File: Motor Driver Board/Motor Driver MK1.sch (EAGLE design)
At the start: 8 parts, among them X1 MAB8SH, X2 MAB8SH, X3 MAB8SH, X4 MAB8SH

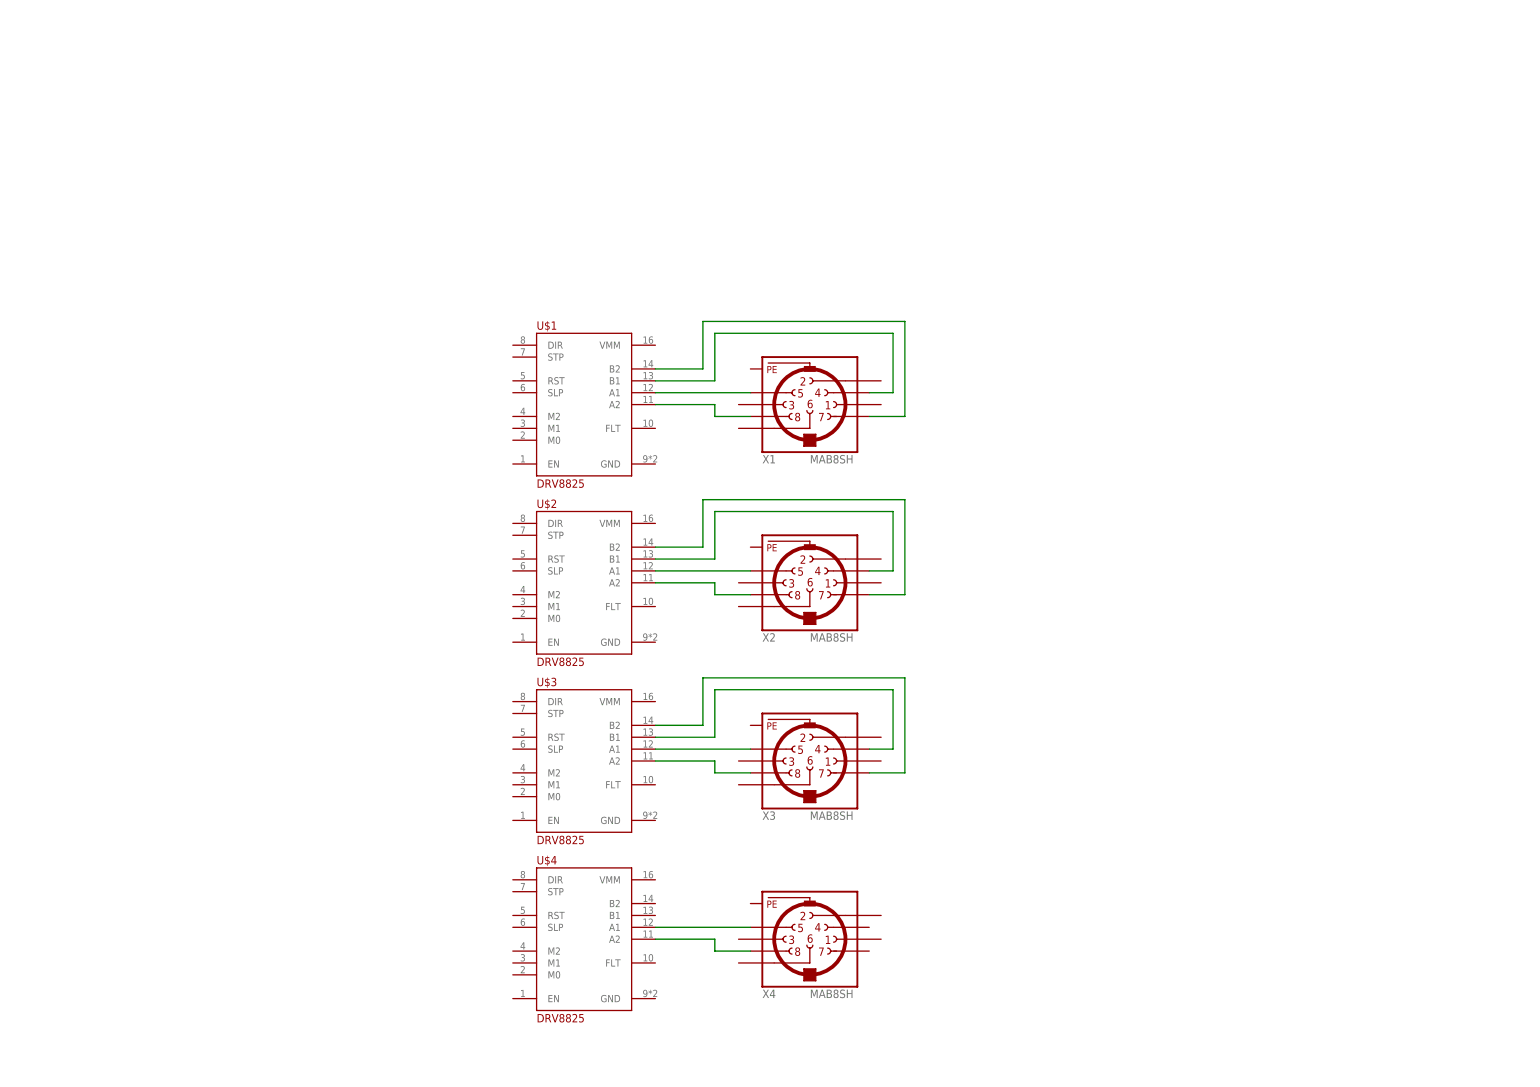
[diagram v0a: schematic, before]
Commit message: finished up schematic
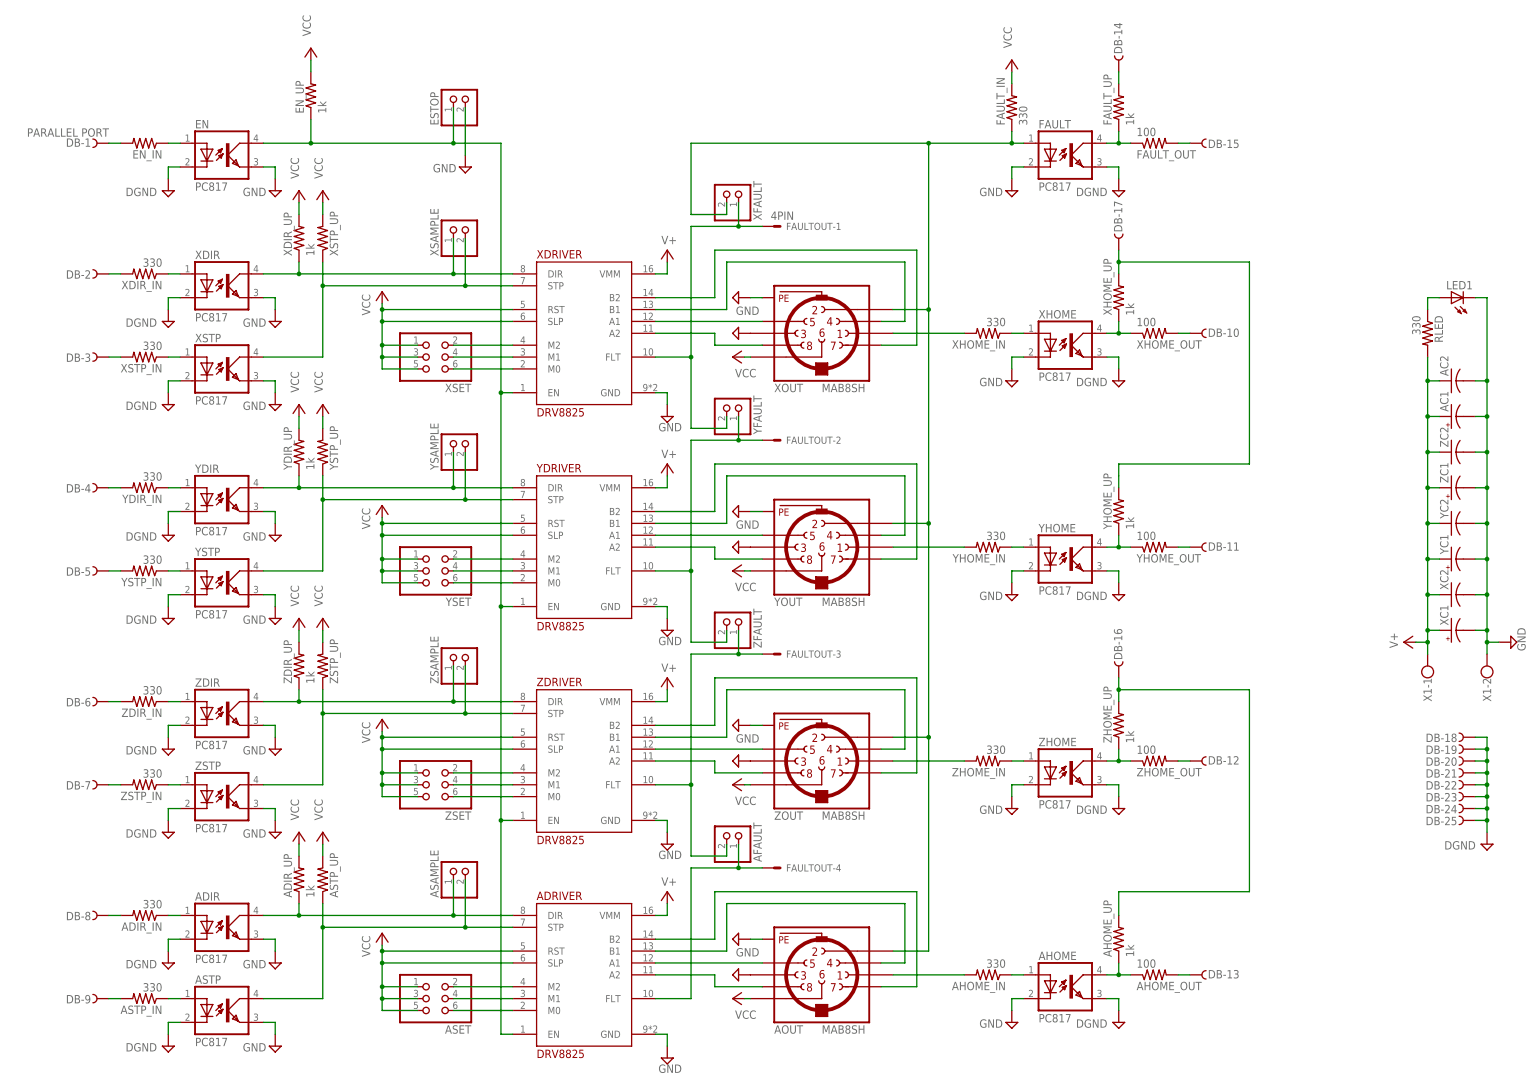
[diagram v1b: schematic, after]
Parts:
- removed U$1, U$2, U$4: DRV8825, CNC-Interface:DRV8825
- removed X2, X3, X4: MAB8SH, con-hirschmann:MAB8SH
- added AC1, XC1, YC1, ZC1: (no value), rcl:CPOL-USSANYO_SMD_F12
- added AC2, XC2, YC2, ZC2: (no value), rcl:C-USC0805
- added ADIR, AHOME, ASTP, EN, FAULT, XDIR, XHOME, XSTP, YDIR, YHOME, YSTP, ZDIR, ZHOME, ZSTP: PC817, optocoupler:PC817
- added ADIR_IN, AHOME_IN, ASTP_IN, FAULT_IN, RLED, XDIR_IN, XHOME_IN, XSTP_IN, YDIR_IN, YHOME_IN, YSTP_IN, ZDIR_IN, ZHOME_IN, ZSTP_IN: 330, resistor:R-US_R0805
- added ADIR_UP, AHOME_UP, EN_UP, FAULT_UP, XDIR_UP, XHOME_UP, YDIR_UP, YHOME_UP, ZDIR_UP, ZHOME_UP: 1k, resistor:R-US_R0805
- added ADRIVER, XDRIVER, YDRIVER: DRV8825, CNC-Interface:DRV8825
- added AFAULT, ASAMPLE, ESTOP, XFAULT, XSAMPLE, YFAULT, YSAMPLE, ZFAULT, ZSAMPLE: (no value), pinhead:PINHD-1X2
- added AHOME_OUT, FAULT_OUT, XHOME_OUT, YHOME_OUT, ZHOME_OUT: 100, resistor:R-US_R0805
- added AOUT, XOUT, YOUT, ZOUT: MAB8SH, con-hirschmann:MAB8SH
- added ASET, XSET, YSET, ZSET: (no value), pinhead:PINHD-2X3
- added ASTP_UP, EN_IN, XSTP_UP, YSTP_UP, ZSTP_UP: (no value), resistor:R-US_R0805
- added DB: PARALLEL PORT, con-thomas-betts:D-SUB25-H2R25ST
- added FAULTOUT: 4PIN, con-molex:22-23-2041
- added LED1: (no value), led:LEDCHIP-LED0805
- X1: value MAB8SH -> (none); device con-hirschmann:MAB8SH -> con-wago-500:W237-102
- renumbered U$3 to ZDRIVER
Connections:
- new net ASTP_UP: ADRIVER.STP, ASAMPLE.2, ASTP.COL, ASTP_UP.1
- new net DGND: ADIR.C, AHOME.EMIT, ASTP.C, DB-18.F, DB-19.F, DB-20.F, DB-21.F, DB-22.F, DB-23.F, DB-24.F, DB-25.F, EN.C, FAULT.EMIT, XDIR.C, XHOME.EMIT, XSTP.C, YDIR.C, YHOME.EMIT, YSTP.C, ZDIR.C, ZHOME.EMIT, ZSTP.C
- new net GND: AC1.-, AC2.2, ADIR.EMIT, ADRIVER.GND, AHOME.C, AOUT.3, AOUT.PE, ASTP.EMIT, EN.EMIT, ESTOP.2, FAULT.C, LED1.C, X1-2.KL, XC1.-, XC2.2, XDIR.EMIT, XDRIVER.GND, XHOME.C, XOUT.3, XOUT.PE, XSTP.EMIT, YC1.-, YC2.2, YDIR.EMIT, YDRIVER.GND, YHOME.C, YOUT.3, YOUT.PE, YSTP.EMIT, ZC1.-, ZC2.2, ZDIR.EMIT, ZDRIVER.GND, ZHOME.C, ZOUT.3, ZOUT.PE, ZSTP.EMIT
- new net N$15: ADRIVER.B1, AOUT.4
- new net N$16: ADRIVER.B2, AOUT.7
- new net N$17: LED1.A, RLED.1
- new net N$18: XDRIVER.STP, XSAMPLE.2, XSTP.COL, XSTP_UP.1
- new net N$19: XDRIVER.M2, XSET.2
- new net N$20: XDRIVER.M1, XSET.4
- new net N$21: XDRIVER.M0, XSET.6
- new net N$22: YDRIVER.M2, YSET.2
- new net N$23: YDRIVER.M1, YSET.4
- new net N$24: YDRIVER.M0, YSET.6
- new net N$25: ADRIVER.M2, ASET.2
- new net N$26: ADRIVER.M1, ASET.4
- new net N$27: ADRIVER.M0, ASET.6
- new net N$28: ZDRIVER.M2, ZSET.2
- new net N$29: ZDRIVER.M1, ZSET.4
- new net N$30: ZDRIVER.M0, ZSET.6
- new net N$33: ADRIVER.EN, EN.COL, EN_UP.1, ESTOP.1, XDRIVER.EN, YDRIVER.EN, ZDRIVER.EN
- new net N$35: EN.A, EN_IN.1
- new net N$37: AFAULT.2, FAULTOUT-3.S, ZDRIVER.FLT, ZFAULT.1
- new net N$38: XDIR.A, XDIR_IN.1
- new net N$39: XSTP.A, XSTP_IN.1
- new net N$40: YDIR.A, YDIR_IN.1
- new net N$41: YSTP.A, YSTP_IN.1
- new net N$42: DB-2.F, XDIR_IN.2
- new net N$43: DB-3.F, XSTP_IN.2
- new net N$44: DB-4.F, YDIR_IN.2
- new net N$45: DB-5.F, YSTP_IN.2
- new net N$46: ZSTP.A, ZSTP_IN.1
- new net N$47: ZDIR.A, ZDIR_IN.1
- new net N$48: DB-6.F, ZDIR_IN.2
- new net N$49: DB-7.F, ZSTP_IN.2
- new net N$50: ADIR.A, ADIR_IN.1
- new net N$51: ADIR_IN.2, DB-8.F
- new net N$52: ASTP_IN.2, DB-9.F
- new net N$53: ASTP.A, ASTP_IN.1
- new net N$54: DB-1.F, EN_IN.2
- new net N$55: DB-10.F, XHOME_OUT.2
- new net N$57: ADIR.COL, ADIR_UP.1, ADRIVER.DIR, ASAMPLE.1
- new net N$58: FAULT.COL, FAULT_OUT.1, FAULT_UP.1
- new net N$59: DB-15.F, FAULT_OUT.2
- new net N$60: FAULTOUT-1.S, XDRIVER.FLT, XFAULT.1, YFAULT.2
- new net N$61: FAULTOUT-2.S, YDRIVER.FLT, YFAULT.1, ZFAULT.2
- new net N$62: ADRIVER.FLT, AFAULT.1, FAULTOUT-4.S
- new net N$63: AOUT.2, FAULT.A, FAULT_IN.1, XFAULT.2, XOUT.2, YOUT.2, ZOUT.2
- new net N$64: XHOME_IN.2, XOUT.1
- new net N$65: YHOME_IN.2, YOUT.1
- new net N$66: ZHOME_IN.2, ZOUT.1
- new net N$67: AHOME_IN.2, AOUT.1
- new net N$69: YHOME.COL, YHOME_OUT.1, YHOME_UP.1
- new net N$70: XHOME.A, XHOME_IN.1
- new net N$71: YHOME.A, YHOME_IN.1
- new net N$72: ZHOME.A, ZHOME_IN.1
- new net N$73: AHOME.A, AHOME_IN.1
- new net N$74: DB-11.F, YHOME_OUT.2
- new net N$75: ZHOME.COL, ZHOME_OUT.1, ZHOME_UP.1
- new net N$76: DB-12.F, ZHOME_OUT.2
- new net N$77: AHOME_OUT.2, DB-13.F
- new net N$78: AHOME.COL, AHOME_OUT.1, AHOME_UP.1
- new net N$79: DB-14.F, FAULT_UP.2
- new net N$80: DB-17.F, XHOME_UP.2, YHOME_UP.2
- new net N$82: AHOME_UP.2, DB-16.F, ZHOME_UP.2
- new net V+: AC1.+, AC2.1, ADRIVER.VMM, RLED.2, X1-1.KL, XC1.+, XC2.1, XDRIVER.VMM, YC1.+, YC2.1, YDRIVER.VMM, ZC1.+, ZC2.1, ZDRIVER.VMM
- new net VCC: ADIR_UP.2, ADRIVER.RST, ADRIVER.SLP, AOUT.6, ASET.1, ASET.3, ASET.5, ASTP_UP.2, EN_UP.2, FAULT_IN.2, XDIR_UP.2, XDRIVER.RST, XDRIVER.SLP, XOUT.6, XSET.1, XSET.3, XSET.5, XSTP_UP.2, YDIR_UP.2, YDRIVER.RST, YDRIVER.SLP, YOUT.6, YSET.1, YSET.3, YSET.5, YSTP_UP.2, ZDIR_UP.2, ZDRIVER.RST, ZDRIVER.SLP, ZOUT.6, ZSET.1, ZSET.3, ZSET.5, ZSTP_UP.2
- new net XHOME_UP: XHOME.COL, XHOME_OUT.1, XHOME_UP.1
- new net XSAMPLE: XDIR.COL, XDIR_UP.1, XDRIVER.DIR, XSAMPLE.1
- new net YDIR: YDIR.COL, YDIR_UP.1, YDRIVER.DIR, YSAMPLE.1
- new net YSTP: YDRIVER.STP, YSAMPLE.2, YSTP.COL, YSTP_UP.1
- new net ZDIR: ZDIR.COL, ZDIR_UP.1, ZDRIVER.DIR, ZSAMPLE.1
- new net ZSTP: ZDRIVER.STP, ZSAMPLE.2, ZSTP.COL, ZSTP_UP.1
- net N$1: now also XDRIVER.A2, XOUT.8; no longer U$1.A2, X1.8
- net N$10: now also ZOUT.5; no longer X3.5
- net N$11: now also ZOUT.8; no longer X3.8
- net N$12: now also ZOUT.4; no longer X3.4
- net N$13: now also ZOUT.7; no longer X3.7
- net N$14: now also ADRIVER.A2, AOUT.8; no longer U$4.A2, X4.8
- net N$2: now also XDRIVER.A1, XOUT.5; no longer U$1.A1, X1.5
- net N$3: now also XDRIVER.B1, XOUT.4; no longer U$1.B1, X1.4
- net N$4: now also XDRIVER.B2, XOUT.7; no longer U$1.B2, X1.7
- net N$5: now also ADRIVER.A1, AOUT.5; no longer U$4.A1, X4.5
- net N$6: now also YDRIVER.A1, YOUT.5; no longer U$2.A1, X2.5
- net N$7: now also YDRIVER.A2, YOUT.8; no longer U$2.A2, X2.8
- net N$8: now also YDRIVER.B1, YOUT.4; no longer U$2.B1, X2.4
- net N$9: now also YDRIVER.B2, YOUT.7; no longer U$2.B2, X2.7
